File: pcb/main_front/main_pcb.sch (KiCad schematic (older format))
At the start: 31 parts, among them J1 AVR-ISP-6, J2 USB_C_Receptacle_USB2.0, Q1 Q_NMOS_DGS, SW1 RESET, SW2 BOOT, SW3 BL_STEP, U1 ATmega32-16PU, Y1 Crystal

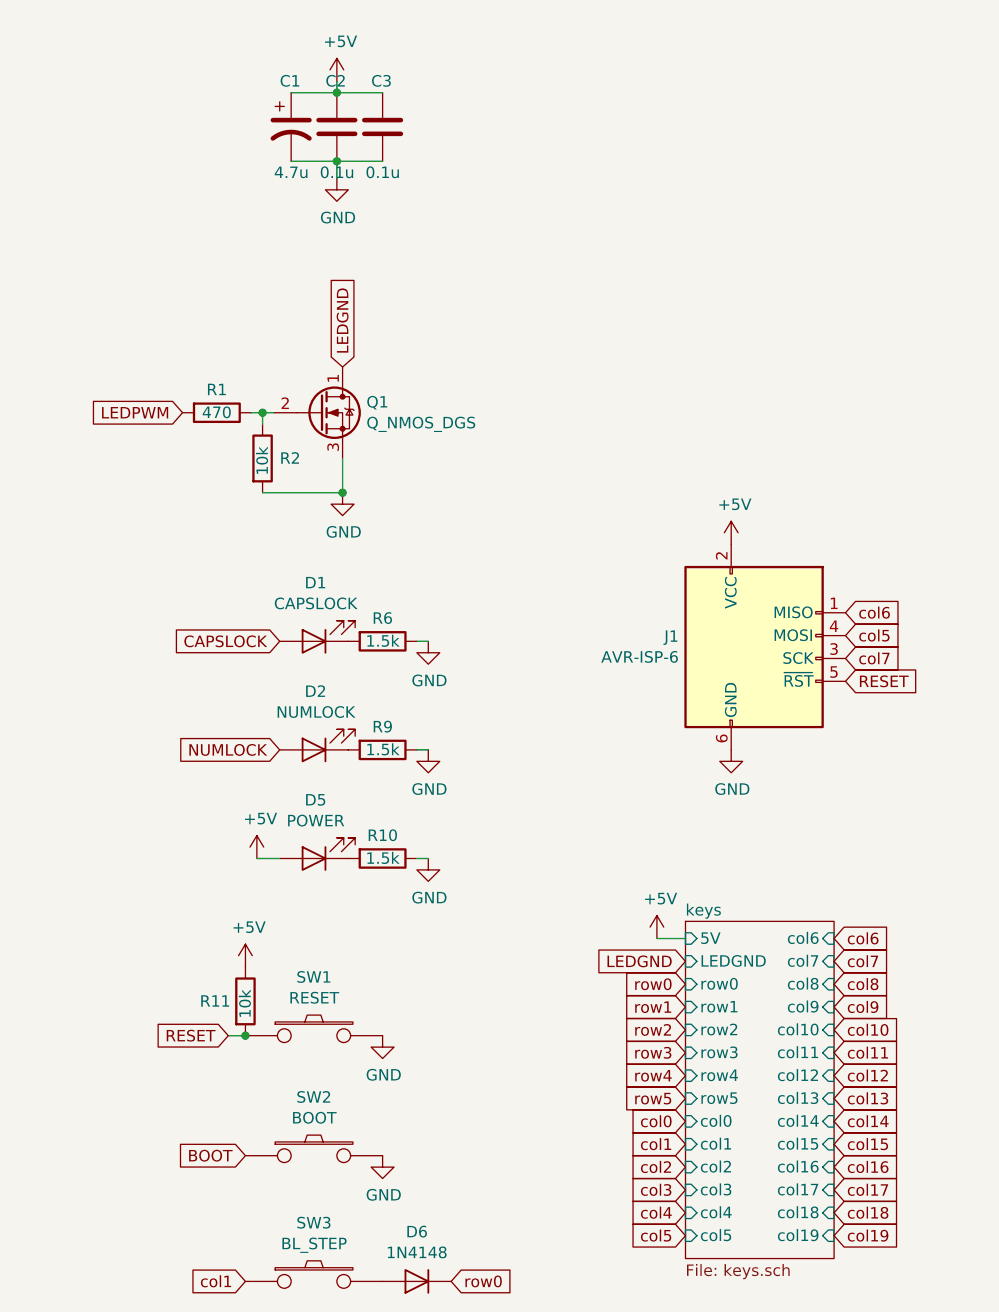
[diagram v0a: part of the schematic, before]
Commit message: Begin revised PCB layout
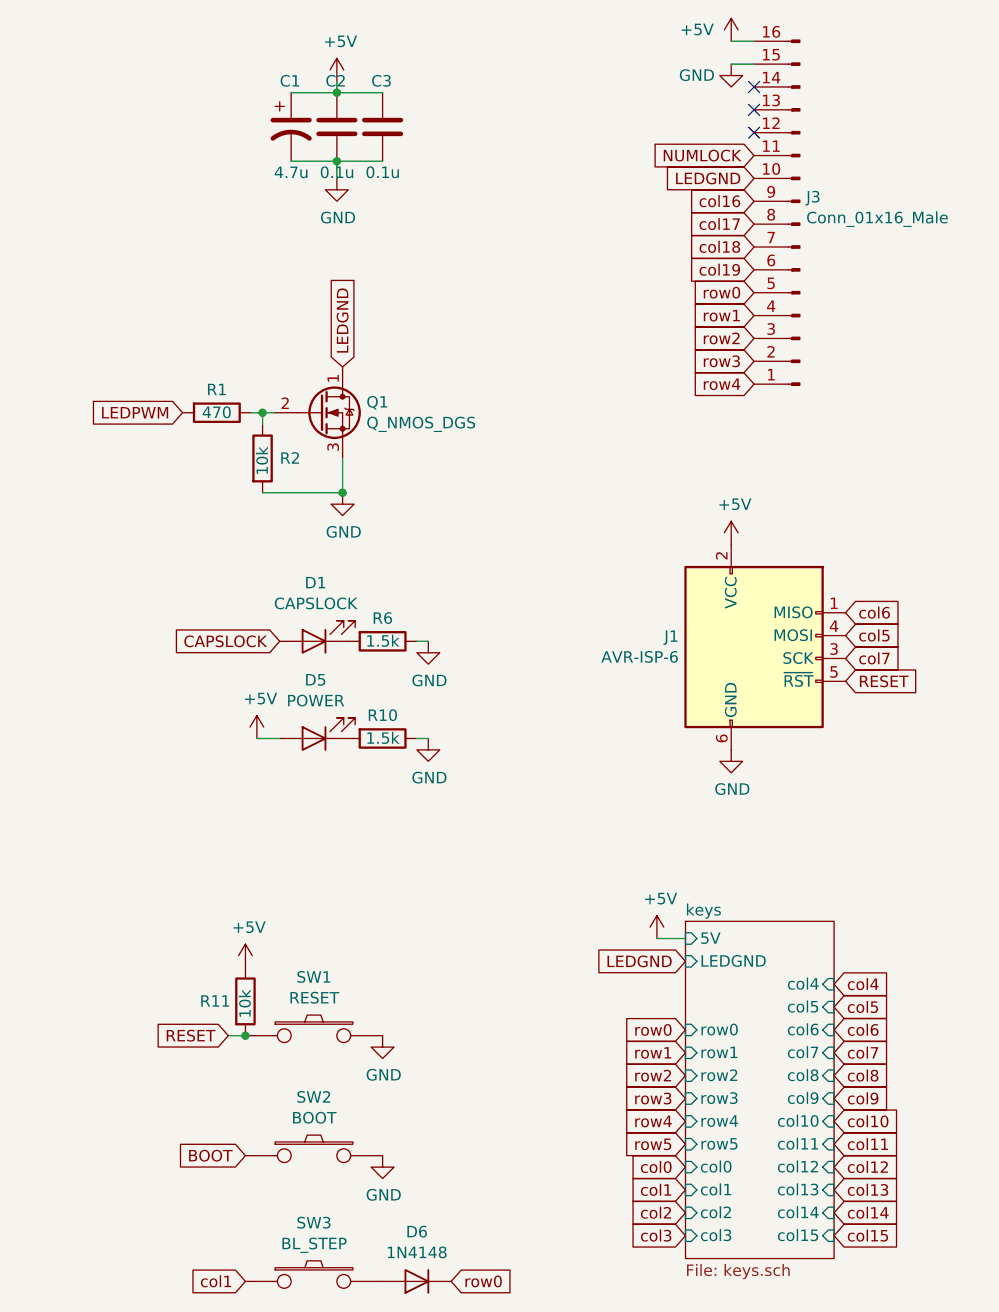
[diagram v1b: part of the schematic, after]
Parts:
- removed D2: NUMLOCK, LED_THT:LED_D3.0mm_Clear, symbol Device:LED
- removed R9: 1.5k, Resistor_THT:R_Axial_DIN0204_L3.6mm_D1.6mm_P7.62mm_Horizontal, symbol Device:R
- added J3: Conn_01x16_Male, Connector_PinHeader_2.54mm:PinHeader_2x08_P2.54mm_Horizontal, symbol Connector:Conn_01x16_Male
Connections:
- net +5V: now also J3.16 (Pin_16)
- net GND: now also J3.15 (Pin_15)
- net LEDGND: now also J3.10 (Pin_10)
- net NUMLOCK: now also J3.11 (Pin_11)
- net col16: now also J3.9 (Pin_9)
- net col17: now also J3.8 (Pin_8)
- net col18: now also J3.7 (Pin_7)
- net col19: now also J3.6 (Pin_6)
- net row0: now also J3.5 (Pin_5)
- net row1: now also J3.4 (Pin_4)
- net row2: now also J3.3 (Pin_3)
- net row3: now also J3.2 (Pin_2)
- net row4: now also J3.1 (Pin_1)
- no-connect marks 3 -> 6
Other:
- moved on the sheet: D5, R10
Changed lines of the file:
@@
 encoding utf-8
 Sheet 1 2
-Title "QBoard - Front"
+Title "QBoard - Main"
 Date "2021-08-26"
 Rev "0"
@@
 L Device:LED D5
 U 1 1 6129195C
-P 7975 4350
-F 0 "D5" H 7968 4095 50  0000 C CNN
-F 1 "POWER" H 7968 4186 50  0000 C CNN
-F 2 "LED_THT:LED_D3.0mm_Clear" H 7975 4350 50  0001 C CNN
-F 3 "~" H 7975 4350 50  0001 C CNN
-	1    7975 4350
+P 7975 3825
+F 0 "D5" H 7968 3570 50  0000 C CNN
+F 1 "POWER" H 7968 3661 50  0000 C CNN
+F 2 "LED_THT:LED_D3.0mm_Clear" H 7975 3825 50  0001 C CNN
+F 3 "~" H 7975 3825 50  0001 C CNN
+	1    7975 3825
 	-1   0    0    1
 $EndComp
@@
 L Device:R R10
 U 1 1 612935EF
-P 8275 4350
-F 0 "R10" V 8175 4350 50  0000 C CNN
-F 1 "1.5k" V 8275 4350 50  0000 C CNN
-F 2 "Resistor_THT:R_Axial_DIN0204_L3.6mm_D1.6mm_P7.62mm_Horizontal" V 8205 4350 50  0001 C CNN
-F 3 "~" H 8275 4350 50  0001 C CNN
-	1    8275 4350
+P 8275 3825
+F 0 "R10" V 8175 3825 50  0000 C CNN
+F 1 "1.5k" V 8275 3825 50  0000 C CNN
+F 2 "Resistor_THT:R_Axial_DIN0204_L3.6mm_D1.6mm_P7.62mm_Horizontal" V 8205 3825 50  0001 C CNN
+F 3 "~" H 8275 3825 50  0001 C CNN
+	1    8275 3825
 	0    1    1    0
 $EndComp
@@
 L power:GND #PWR014
 U 1 1 612967E1
-P 8475 4350
-F 0 "#PWR014" H 8475 4100 50  0001 C CNN
-F 1 "GND" H 8480 4177 50  0000 C CNN
-F 2 "" H 8475 4350 50  0001 C CNN
-F 3 "" H 8475 4350 50  0001 C CNN
-	1    8475 4350
+P 8475 3825
+F 0 "#PWR014" H 8475 3575 50  0001 C CNN
+F 1 "GND" H 8480 3652 50  0000 C CNN
+F 2 "" H 8475 3825 50  0001 C CNN
+F 3 "" H 8475 3825 50  0001 C CNN
+	1    8475 3825
 	1    0    0    -1
 $EndComp
@@
 	8425 3400 8475 3400
 Wire Wire Line
-	8425 4350 8475 4350
+	8425 3825 8475 3825
 $Comp
 L power:+5V #PWR013
 U 1 1 612977F5
-P 7725 4350
-F 0 "#PWR013" H 7725 4200 50  0001 C CNN
-F 1 "+5V" H 7740 4523 50  0000 C CNN
-F 2 "" H 7725 4350 50  0001 C CNN
-F 3 "" H 7725 4350 50  0001 C CNN
-	1    7725 4350
-	1    0    0    -1
-$EndComp
-Wire Wire Line
-	7725 4350 7825 4350
+P 7725 3825
+F 0 "#PWR013" H 7725 3675 50  0001 C CNN
+F 1 "+5V" H 7740 3998 50  0000 C CNN
+F 2 "" H 7725 3825 50  0001 C CNN
+F 3 "" H 7725 3825 50  0001 C CNN
+	1    7725 3825
+	1    0    0    -1
+$EndComp
+Wire Wire Line
+	7725 3825 7825 3825
 $Comp
 L Connector:AVR-ISP-6 J1
@@
 Wire Wire Line
 	9475 4700 9600 4700
-Text GLabel 9600 4900 0    50   Input ~ 0
+Text GLabel 9600 5100 0    50   Input ~ 0
 row0
-Text GLabel 9600 5000 0    50   Input ~ 0
+Text GLabel 9600 5200 0    50   Input ~ 0
 row1
-Text GLabel 9600 5100 0    50   Input ~ 0
+Text GLabel 9600 5300 0    50   Input ~ 0
 row2
-Text GLabel 9600 5200 0    50   Input ~ 0
+Text GLabel 9600 5400 0    50   Input ~ 0
 row3
-Text GLabel 9600 5300 0    50   Input ~ 0
+Text GLabel 9600 5500 0    50   Input ~ 0
 row4
-Text GLabel 9600 5400 0    50   Input ~ 0
+Text GLabel 9600 5600 0    50   Input ~ 0
 row5
 $Sheet
@@
 F2 "5V" I L 9600 4700 50
 F3 "LEDGND" I L 9600 4800 50
-F4 "col0" I L 9600 5500 50
-F5 "col1" I L 9600 5600 50
-F6 "col2" I L 9600 5700 50
-F7 "col3" I L 9600 5800 50
-F8 "col4" I L 9600 5900 50
-F9 "col5" I L 9600 6000 50
-F10 "row0" I L 9600 4900 50
-F11 "row1" I L 9600 5000 50
-F12 "row2" I L 9600 5100 50
-F13 "row3" I L 9600 5200 50
-F14 "row4" I L 9600 5300 50
-F15 "row5" I L 9600 5400 50
-F16 "col6" I R 10250 4700 50
-F17 "col7" I R 10250 4800 50
-F18 "col8" I R 10250 4900 50
-F19 "col9" I R 10250 5000 50
-F20 "col10" I R 10250 5100 50
-F21 "col11" I R 10250 5200 50
-F22 "col12" I R 10250 5300 50
-F23 "col13" I R 10250 5400 50
-F24 "col14" I R 10250 5500 50
-F25 "col15" I R 10250 5600 50
-F26 "col16" I R 10250 5700 50
-F27 "col17" I R 10250 5800 50
-F28 "col18" I R 10250 5900 50
-F29 "col19" I R 10250 6000 50
+F4 "col0" I L 9600 5700 50
+F5 "col1" I L 9600 5800 50
+F6 "col2" I L 9600 5900 50
+F7 "col3" I L 9600 6000 50
+F8 "col4" I R 10250 4900 50
+F9 "col5" I R 10250 5000 50
+F10 "row0" I L 9600 5100 50
+F11 "row1" I L 9600 5200 50
+F12 "row2" I L 9600 5300 50
+F13 "row3" I L 9600 5400 50
+F14 "row4" I L 9600 5500 50
+F15 "row5" I L 9600 5600 50
+F16 "col6" I R 10250 5100 50
+F17 "col7" I R 10250 5200 50
+F18 "col8" I R 10250 5300 50
+F19 "col9" I R 10250 5400 50
+F20 "col10" I R 10250 5500 50
+F21 "col11" I R 10250 5600 50
+F22 "col12" I R 10250 5700 50
+F23 "col13" I R 10250 5800 50
+F24 "col14" I R 10250 5900 50
+F25 "col15" I R 10250 6000 50
 $EndSheet
-Text GLabel 9600 5500 0    50   Input ~ 0
+Text GLabel 9600 5700 0    50   Input ~ 0
 col0
-Text GLabel 9600 5600 0    50   Input ~ 0
+Text GLabel 9600 5800 0    50   Input ~ 0
 col1
-Text GLabel 9600 5700 0    50   Input ~ 0
+Text GLabel 9600 5900 0    50   Input ~ 0
 col2
-Text GLabel 9600 5800 0    50   Input ~ 0
+Text GLabel 9600 6000 0    50   Input ~ 0
 col3
-Text GLabel 9600 5900 0    50   Input ~ 0
+Text GLabel 10250 4900 2    50   Input ~ 0
 col4
-Text GLabel 9600 6000 0    50   Input ~ 0
+Text GLabel 10250 5000 2    50   Input ~ 0
 col5
-Text GLabel 10250 4700 2    50   Input ~ 0
+Text GLabel 10250 5100 2    50   Input ~ 0
 col6
-Text GLabel 10250 4800 2    50   Input ~ 0
+Text GLabel 10250 5200 2    50   Input ~ 0
 col7
-Text GLabel 10250 4900 2    50   Input ~ 0
+Text GLabel 10250 5300 2    50   Input ~ 0
 col8
-Text GLabel 10250 5000 2    50   Input ~ 0
+Text GLabel 10250 5400 2    50   Input ~ 0
 col9
-Text GLabel 10250 5100 2    50   Input ~ 0
+Text GLabel 10250 5500 2    50   Input ~ 0
 col10
-Text GLabel 10250 5200 2    50   Input ~ 0
+Text GLabel 10250 5600 2    50   Input ~ 0
 col11
-Text GLabel 10250 5300 2    50   Input ~ 0
+Text GLabel 10250 5700 2    50   Input ~ 0
 col12
-Text GLabel 10250 5400 2    50   Input ~ 0
+Text GLabel 10250 5800 2    50   Input ~ 0
 col13
-Text GLabel 10250 5500 2    50   Input ~ 0
+Text GLabel 10250 5900 2    50   Input ~ 0
 col14
-Text GLabel 10250 5600 2    50   Input ~ 0
+Text GLabel 10250 6000 2    50   Input ~ 0
 col15
-Text GLabel 10250 5700 2    50   Input ~ 0
-col16
-Text GLabel 10250 5800 2    50   Input ~ 0
-col17
-Text GLabel 10250 5900 2    50   Input ~ 0
-col18
-Text GLabel 10250 6000 2    50   Input ~ 0
-col19
 Text GLabel 6025 3175 2    50   Input ~ 0
 col0
@@
 Text GLabel 6025 5675 2    50   Input ~ 0
 BOOT
-$Comp
-L Device:LED D2
-U 1 1 6132A809
-P 7975 3875
-F 0 "D2" H 7968 3620 50  0000 C CNN
-F 1 "NUMLOCK" H 7968 3711 50  0000 C CNN
-F 2 "LED_THT:LED_D3.0mm_Clear" H 7975 3875 50  0001 C CNN
-F 3 "~" H 7975 3875 50  0001 C CNN
-	1    7975 3875
-	-1   0    0    1
-$EndComp
-$Comp
-L Device:R R9
-U 1 1 6132A80F
-P 8275 3875
-F 0 "R9" V 8175 3875 50  0000 C CNN
-F 1 "1.5k" V 8275 3875 50  0000 C CNN
-F 2 "Resistor_THT:R_Axial_DIN0204_L3.6mm_D1.6mm_P7.62mm_Horizontal" V 8205 3875 50  0001 C CNN
-F 3 "~" H 8275 3875 50  0001 C CNN
-	1    8275 3875
-	0    1    1    0
-$EndComp
-$Comp
-L power:GND #PWR010
-U 1 1 6132A815
-P 8475 3875
-F 0 "#PWR010" H 8475 3625 50  0001 C CNN
-F 1 "GND" H 8480 3702 50  0000 C CNN
-F 2 "" H 8475 3875 50  0001 C CNN
-F 3 "" H 8475 3875 50  0001 C CNN
-	1    8475 3875
-	1    0    0    -1
-$EndComp
-Wire Wire Line
-	8425 3875 8475 3875
-Text GLabel 7825 3875 0    50   Input ~ 0
+Text GLabel 9900 1275 0    50   Input ~ 0
 NUMLOCK
 $Comp
@@
 NoConn ~ 2375 4200
 NoConn ~ 2375 4300
+$Comp
+L Connector:Conn_01x16_Male J3
+U 1 1 61297A0F
+P 10100 1575
+F 0 "J3" H 10072 1457 50  0000 R CNN
+F 1 "Conn_01x16_Male" H 10072 1548 50  0000 R CNN
+F 2 "Connector_PinHeader_2.54mm:PinHeader_2x08_P2.54mm_Horizontal" H 10100 1575 50  0001 C CNN
+F 3 "~" H 10100 1575 50  0001 C CNN
+	1    10100 1575
+	-1   0    0    1
+$EndComp
+$Comp
+L power:+5V #PWR021
+U 1 1 614EDA42
+P 9800 775
+F 0 "#PWR021" H 9800 625 50  0001 C CNN
+F 1 "+5V" H 9650 825 50  0000 C CNN
+F 2 "" H 9800 775 50  0001 C CNN
+F 3 "" H 9800 775 50  0001 C CNN
+	1    9800 775
+	1    0    0    -1
+$EndComp
+Wire Wire Line
+	9800 775  9900 775
+$Comp
+L power:GND #PWR022
+U 1 1 614EF506
+P 9800 875
+F 0 "#PWR022" H 9800 625 50  0001 C CNN
+F 1 "GND" H 9650 825 50  0000 C CNN
+F 2 "" H 9800 875 50  0001 C CNN
+F 3 "" H 9800 875 50  0001 C CNN
+	1    9800 875
+	1    0    0    -1
+$EndComp
+Wire Wire Line
+	9800 875  9900 875
+NoConn ~ 9900 975
+NoConn ~ 9900 1075
+NoConn ~ 9900 1175
+Text GLabel 9900 1375 0    50   Input ~ 0
+LEDGND
+Text GLabel 9900 1475 0    50   Input ~ 0
+col16
+Text GLabel 9900 1575 0    50   Input ~ 0
+col17
+Text GLabel 9900 1675 0    50   Input ~ 0
+col18
+Text GLabel 9900 1775 0    50   Input ~ 0
+col19
+Text GLabel 9900 1875 0    50   Input ~ 0
+row0
+Text GLabel 9900 1975 0    50   Input ~ 0
+row1
+Text GLabel 9900 2075 0    50   Input ~ 0
+row2
+Text GLabel 9900 2175 0    50   Input ~ 0
+row3
+Text GLabel 9900 2275 0    50   Input ~ 0
+row4
 $EndSCHEMATC
